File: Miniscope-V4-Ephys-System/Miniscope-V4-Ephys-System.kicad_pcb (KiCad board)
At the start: 4 copper layers, 24.2 x 15.5 mm, 67 parts, among them J1 34 Circuit Slimslack Connector, J10 Conn_01x01, J11 Conn_01x01, J12 Conn_01x01, J13 Conn_01x01, J14 Conn_01x05, J15 Conn_01x01, J16 Conn_01x01, J17 Conn_01x01, J18 Conn_01x01, J19 Conn_01x01, J2 Conn_01x01, J20 Conn_01x01, J21 Conn_01x01, J22 Conn_01x01, J23 Conn_01x01, J24 Conn_01x01, J25 Conn_01x01, J26 Conn_01x01, J27 Conn_01x01, J28 Conn_01x01, J3 Conn_01x01, J4 Conn_01x01, J5 Conn_01x01, J6 Conn_01x01, J7 Conn_01x01, J8 Conn_01x01, J9 Conn_01x01, Q1 MMBT3904LP-7B, U1 RHD2132, U2 TXB0304RUT, U3 MCP1711T-30I/5X, U4 ATSAME70N21A-CN, U5 MCP1711T-18I/5X, Y1 SMD_CRYSTAL

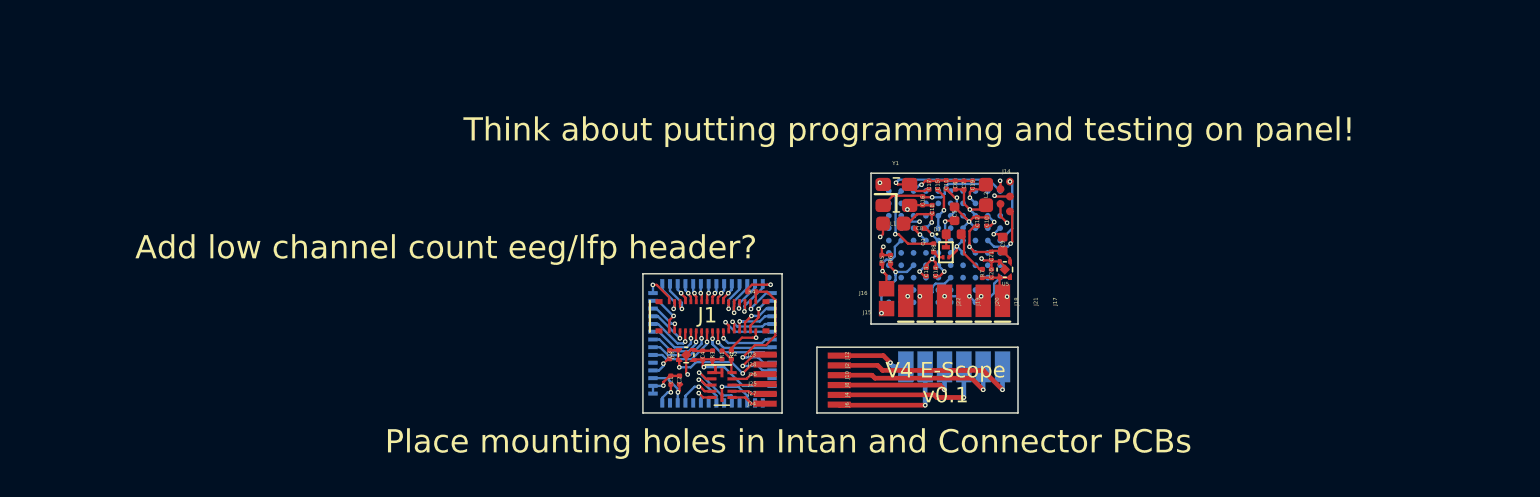
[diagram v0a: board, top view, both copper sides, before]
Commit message: Add files via upload
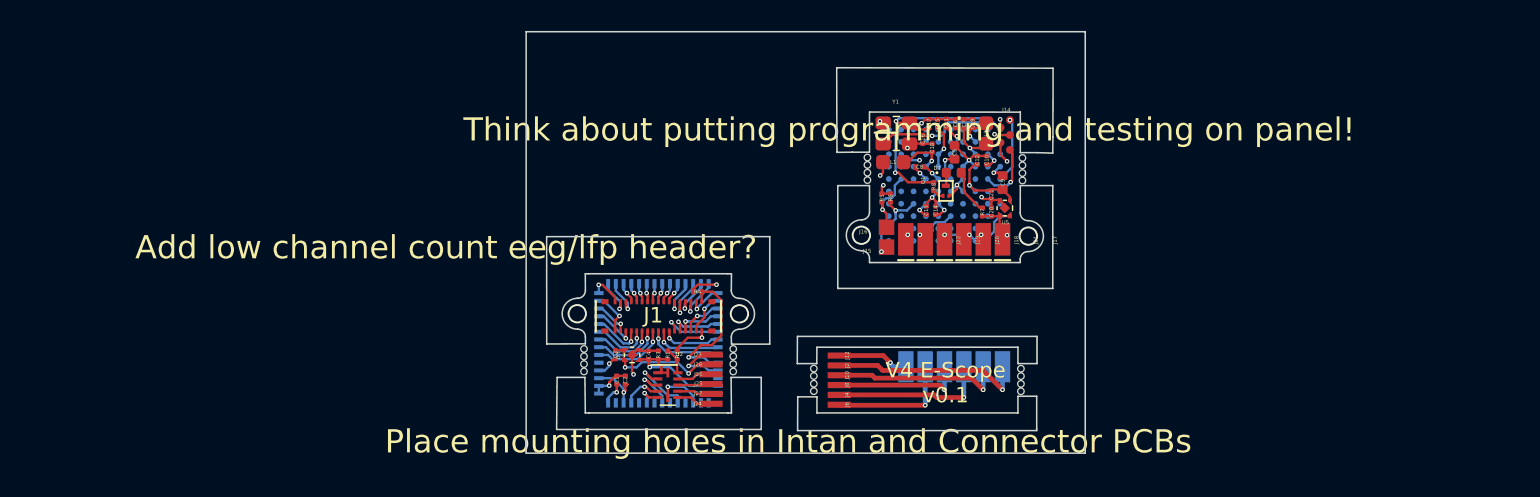
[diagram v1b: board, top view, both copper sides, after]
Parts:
- moved C10 3.98 mm to (129.0, 118.7)
- moved C12 3.98 mm to (128.4, 118.7)
- moved C13 3.98 mm to (125.1, 121.9)
- moved C14 3.98 mm to (125.7, 121.9)
- moved C15 3.98 mm to (125.8, 116.3)
- moved C17 3.98 mm to (125.2, 116.3)
- moved C18 3.98 mm to (125.5, 117.9)
- moved C19 3.98 mm to (128.1, 116.3)
- moved C6 3.98 mm to (126.9, 116.3)
- moved C7 3.98 mm to (127.5, 116.3)
- moved C8 3.98 mm to (124.6, 119.1)
- moved C9 3.98 mm to (130.0, 120.1)
- moved D1 3.98 mm to (126.8, 119.5)
- moved J14 3.98 mm to (130.5, 116.1)
- moved L1 3.98 mm to (122.9, 118.8)
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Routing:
- net (no net): vias 0 -> 4
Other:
- board size 24.2 x 15.5 mm -> 36.1 x 27.2 mm

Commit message: Revert "pcb file updated"
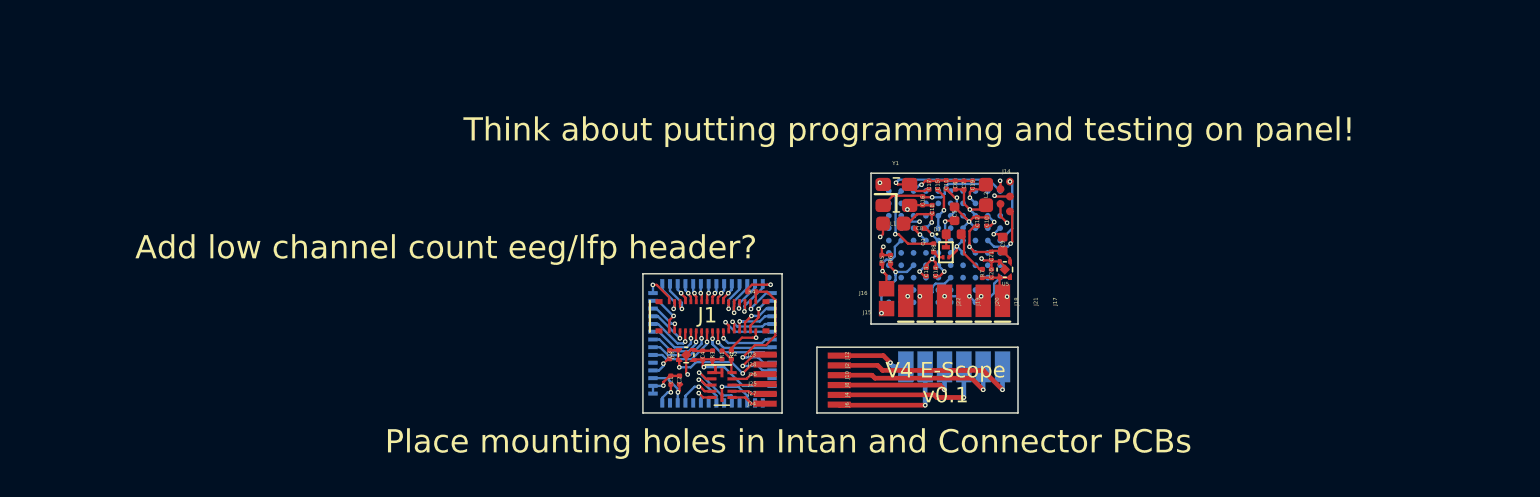
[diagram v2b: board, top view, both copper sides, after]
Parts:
- moved C10 3.98 mm to (129.0, 122.6)
- moved C12 3.98 mm to (128.4, 122.6)
- moved C13 3.98 mm to (125.1, 125.9)
- moved C14 3.98 mm to (125.7, 125.9)
- moved C15 3.98 mm to (125.8, 120.3)
- moved C17 3.98 mm to (125.2, 120.3)
- moved C18 3.98 mm to (125.5, 121.8)
- moved C19 3.98 mm to (128.1, 120.3)
- moved C6 3.98 mm to (126.9, 120.3)
- moved C7 3.98 mm to (127.5, 120.3)
- moved C8 3.98 mm to (124.6, 123.1)
- moved C9 3.98 mm to (130.0, 124.1)
- moved D1 3.98 mm to (126.8, 123.4)
- moved J14 3.98 mm to (130.5, 120.0)
- moved L1 3.98 mm to (122.9, 122.8)
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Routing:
- net (no net): vias 4 -> 0
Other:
- board size 36.1 x 27.2 mm -> 24.2 x 15.5 mm
